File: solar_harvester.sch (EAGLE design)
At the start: 36 parts, among them U1 BQ25505, U2 TPS61322XA, U3 TPS61322XA, U4 MAX17040, U5 INA226, U6 DMP3085LSD

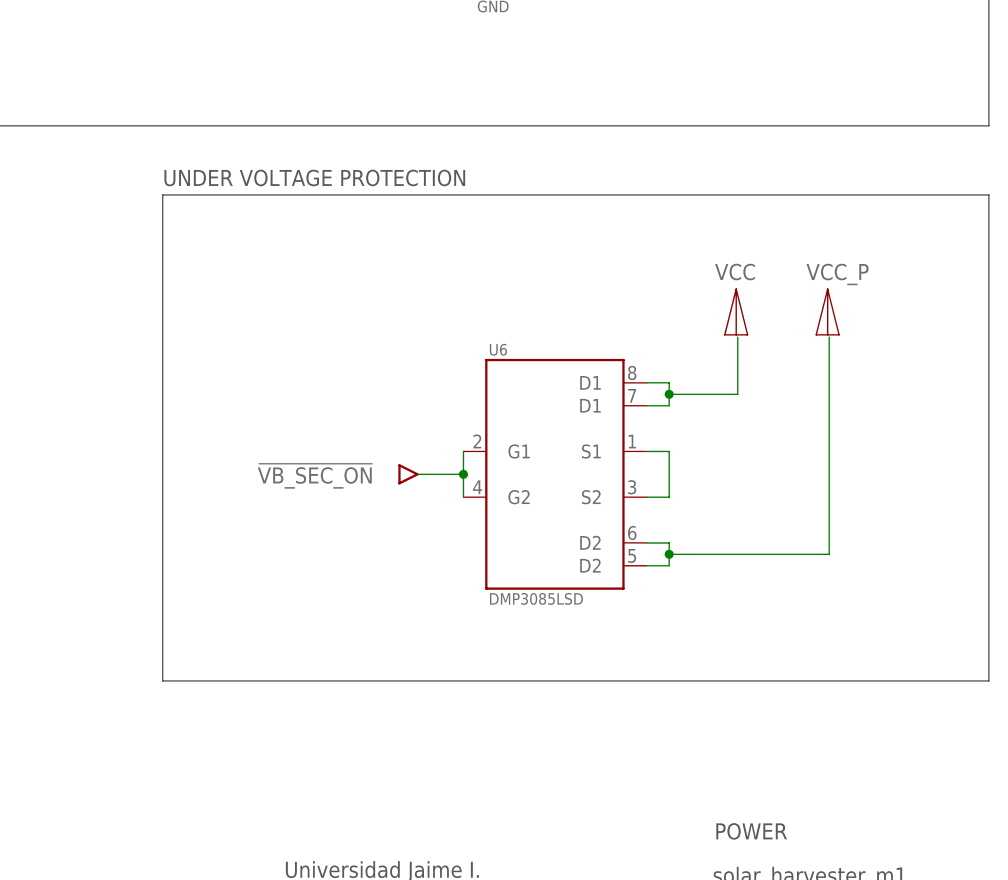
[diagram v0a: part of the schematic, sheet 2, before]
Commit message: uv routed done
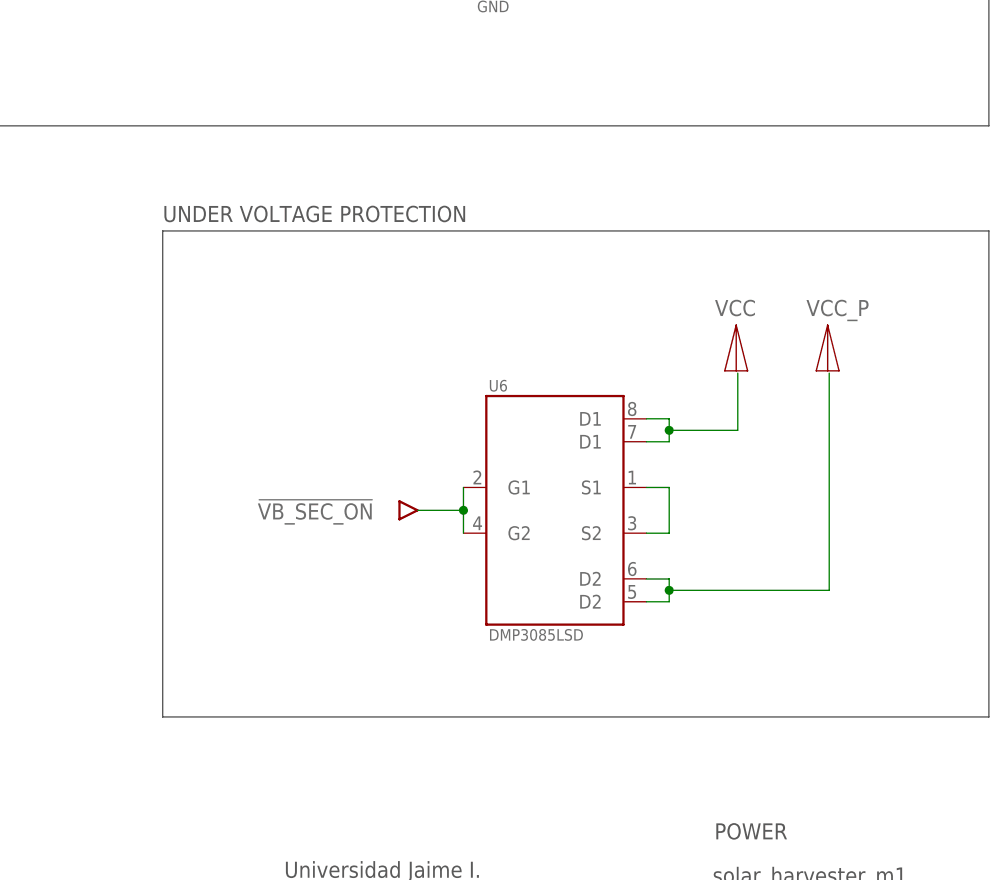
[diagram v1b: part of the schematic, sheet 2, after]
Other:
- moved on the sheet: U6
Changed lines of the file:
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@@
 Architecture) Research Group</text>
 <text x="217.4" y="10.6" size="1.778" layer="97">Vladislav Rykov</text>
-<wire x1="247.8" y1="92" x2="247.8" y2="38" width="0.1524" layer="97"/>
-<wire x1="247.8" y1="38" x2="156" y2="38" width="0.1524" layer="97"/>
-<wire x1="156" y1="38" x2="156" y2="92" width="0.1524" layer="97"/>
-<wire x1="156" y1="92" x2="247.8" y2="92" width="0.1524" layer="97"/>
-<text x="156" y="93" size="1.778" layer="97">UNDER VOLTAGE PROTECTION</text>
+<wire x1="247.8" y1="88" x2="247.8" y2="34" width="0.1524" layer="97"/>
+<wire x1="247.8" y1="34" x2="156" y2="34" width="0.1524" layer="97"/>
+<wire x1="156" y1="34" x2="156" y2="88" width="0.1524" layer="97"/>
+<wire x1="156" y1="88" x2="247.8" y2="88" width="0.1524" layer="97"/>
+<text x="156" y="89" size="1.778" layer="97">UNDER VOLTAGE PROTECTION</text>
 </plain>
 <instances>
@@
 <instance part="U$23" gate="G$1" x="75.518" y="156.718" smashed="yes"/>
 <instance part="U$30" gate="G$1" x="172.292" y="149.352" smashed="yes"/>
-<instance part="U6" gate="G$1" x="199.58" y="60.96" smashed="yes">
-<attribute name="NAME" x="192.214" y="74.168" size="1.27" layer="95"/>
-<attribute name="VALUE" x="192.214" y="46.482" size="1.27" layer="96"/>
-</instance>
-<instance part="U$32" gate="G$1" x="182.308" y="60.96" smashed="yes" rot="R270"/>
-<instance part="U$33" gate="G$1" x="219.726" y="76.454" smashed="yes"/>
-<instance part="U$34" gate="G$1" x="229.886" y="76.454" smashed="yes"/>
+<instance part="U6" gate="G$1" x="199.58" y="56.96" smashed="yes">
+<attribute name="NAME" x="192.214" y="70.168" size="1.27" layer="95"/>
+<attribute name="VALUE" x="192.214" y="42.482" size="1.27" layer="96"/>
+</instance>
+<instance part="U$32" gate="G$1" x="182.308" y="56.96" smashed="yes" rot="R270"/>
+<instance part="U$33" gate="G$1" x="219.726" y="72.454" smashed="yes"/>
+<instance part="U$34" gate="G$1" x="229.886" y="72.454" smashed="yes"/>
 </instances>
 <busses>
@@
 <segment>
 <pinref part="U6" gate="G$1" pin="D1@1"/>
-<wire x1="209.74" y1="71.12" x2="212.28" y2="71.12" width="0.1524" layer="91"/>
-<wire x1="212.28" y1="71.12" x2="212.28" y2="69.85" width="0.1524" layer="91"/>
+<wire x1="209.74" y1="67.12" x2="212.28" y2="67.12" width="0.1524" layer="91"/>
+<wire x1="212.28" y1="67.12" x2="212.28" y2="65.85" width="0.1524" layer="91"/>
 <pinref part="U6" gate="G$1" pin="D1@2"/>
-<wire x1="212.28" y1="69.85" x2="212.28" y2="68.58" width="0.1524" layer="91"/>
-<wire x1="212.28" y1="68.58" x2="209.74" y2="68.58" width="0.1524" layer="91"/>
-<junction x="212.28" y="69.85"/>
-<label x="217.36" y="82.55" size="1.778" layer="95"/>
-<wire x1="212.28" y1="69.85" x2="219.9" y2="69.85" width="0.1524" layer="91"/>
-<wire x1="219.9" y1="69.85" x2="219.9" y2="76.2" width="0.1524" layer="91"/>
+<wire x1="212.28" y1="65.85" x2="212.28" y2="64.58" width="0.1524" layer="91"/>
+<wire x1="212.28" y1="64.58" x2="209.74" y2="64.58" width="0.1524" layer="91"/>
+<junction x="212.28" y="65.85"/>
+<label x="217.36" y="78.55" size="1.778" layer="95"/>
+<wire x1="212.28" y1="65.85" x2="219.9" y2="65.85" width="0.1524" layer="91"/>
+<wire x1="219.9" y1="65.85" x2="219.9" y2="72.2" width="0.1524" layer="91"/>
 </segment>
 </net>
@@
 <segment>
 <pinref part="U6" gate="G$1" pin="D2@1"/>
-<wire x1="209.74" y1="53.34" x2="212.28" y2="53.34" width="0.1524" layer="91"/>
+<wire x1="209.74" y1="49.34" x2="212.28" y2="49.34" width="0.1524" layer="91"/>
 <pinref part="U6" gate="G$1" pin="D2@2"/>
-<wire x1="212.28" y1="53.34" x2="212.28" y2="52.07" width="0.1524" layer="91"/>
-<wire x1="212.28" y1="52.07" x2="212.28" y2="50.8" width="0.1524" layer="91"/>
-<wire x1="212.28" y1="50.8" x2="209.74" y2="50.8" width="0.1524" layer="91"/>
-<junction x="212.28" y="52.07"/>
-<label x="227.52" y="82.55" size="1.778" layer="95"/>
-<wire x1="212.28" y1="52.07" x2="230.06" y2="52.07" width="0.1524" layer="91"/>
-<wire x1="230.06" y1="52.07" x2="230.06" y2="76.2" width="0.1524" layer="91"/>
+<wire x1="212.28" y1="49.34" x2="212.28" y2="48.07" width="0.1524" layer="91"/>
+<wire x1="212.28" y1="48.07" x2="212.28" y2="46.8" width="0.1524" layer="91"/>
+<wire x1="212.28" y1="46.8" x2="209.74" y2="46.8" width="0.1524" layer="91"/>
+<junction x="212.28" y="48.07"/>
+<label x="227.52" y="78.55" size="1.778" layer="95"/>
+<wire x1="212.28" y1="48.07" x2="230.06" y2="48.07" width="0.1524" layer="91"/>
+<wire x1="230.06" y1="48.07" x2="230.06" y2="72.2" width="0.1524" layer="91"/>
 </segment>
 </net>
@@
 <segment>
 <pinref part="U6" gate="G$1" pin="S2"/>
-<wire x1="209.74" y1="58.42" x2="212.28" y2="58.42" width="0.1524" layer="91"/>
-<wire x1="212.28" y1="58.42" x2="212.28" y2="63.5" width="0.1524" layer="91"/>
+<wire x1="209.74" y1="54.42" x2="212.28" y2="54.42" width="0.1524" layer="91"/>
+<wire x1="212.28" y1="54.42" x2="212.28" y2="59.5" width="0.1524" layer="91"/>
 <pinref part="U6" gate="G$1" pin="S1"/>
-<wire x1="212.28" y1="63.5" x2="209.74" y2="63.5" width="0.1524" layer="91"/>
+<wire x1="212.28" y1="59.5" x2="209.74" y2="59.5" width="0.1524" layer="91"/>
 </segment>
 </net>
@@
 <pinref part="U6" gate="G$1" pin="G1"/>
 <pinref part="U6" gate="G$1" pin="G2"/>
-<wire x1="189.42" y1="63.5" x2="189.42" y2="60.96" width="0.1524" layer="91"/>
-<wire x1="189.42" y1="60.96" x2="189.42" y2="58.42" width="0.1524" layer="91"/>
-<wire x1="189.42" y1="60.96" x2="184.34" y2="60.96" width="0.1524" layer="91"/>
-<junction x="189.42" y="60.96"/>
-<label x="166.56" y="59.944" size="1.778" layer="95"/>
-</segment>
-</net>
+<wire x1="189.42" y1="59.5" x2="189.42" y2="56.96" width="0.1524" layer="91"/>
+<wire x1="189.42" y1="56.96" x2="189.42" y2="54.42" width="0.1524" layer="91"/>
+<wire x1="189.42" y1="56.96" x2="184.34" y2="56.96" width="0.1524" layer="91"/>
+<junction x="189.42" y="56.96"/>
+<label x="166.56" y="55.944" size="1.778" layer="95"/>
+</segment>
+</net>
